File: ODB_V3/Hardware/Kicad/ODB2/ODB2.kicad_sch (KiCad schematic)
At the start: 95 parts, among them U1 STM32F412ZGTx, Y1 ABM8G-25.000MHZ-18-D2Y-T

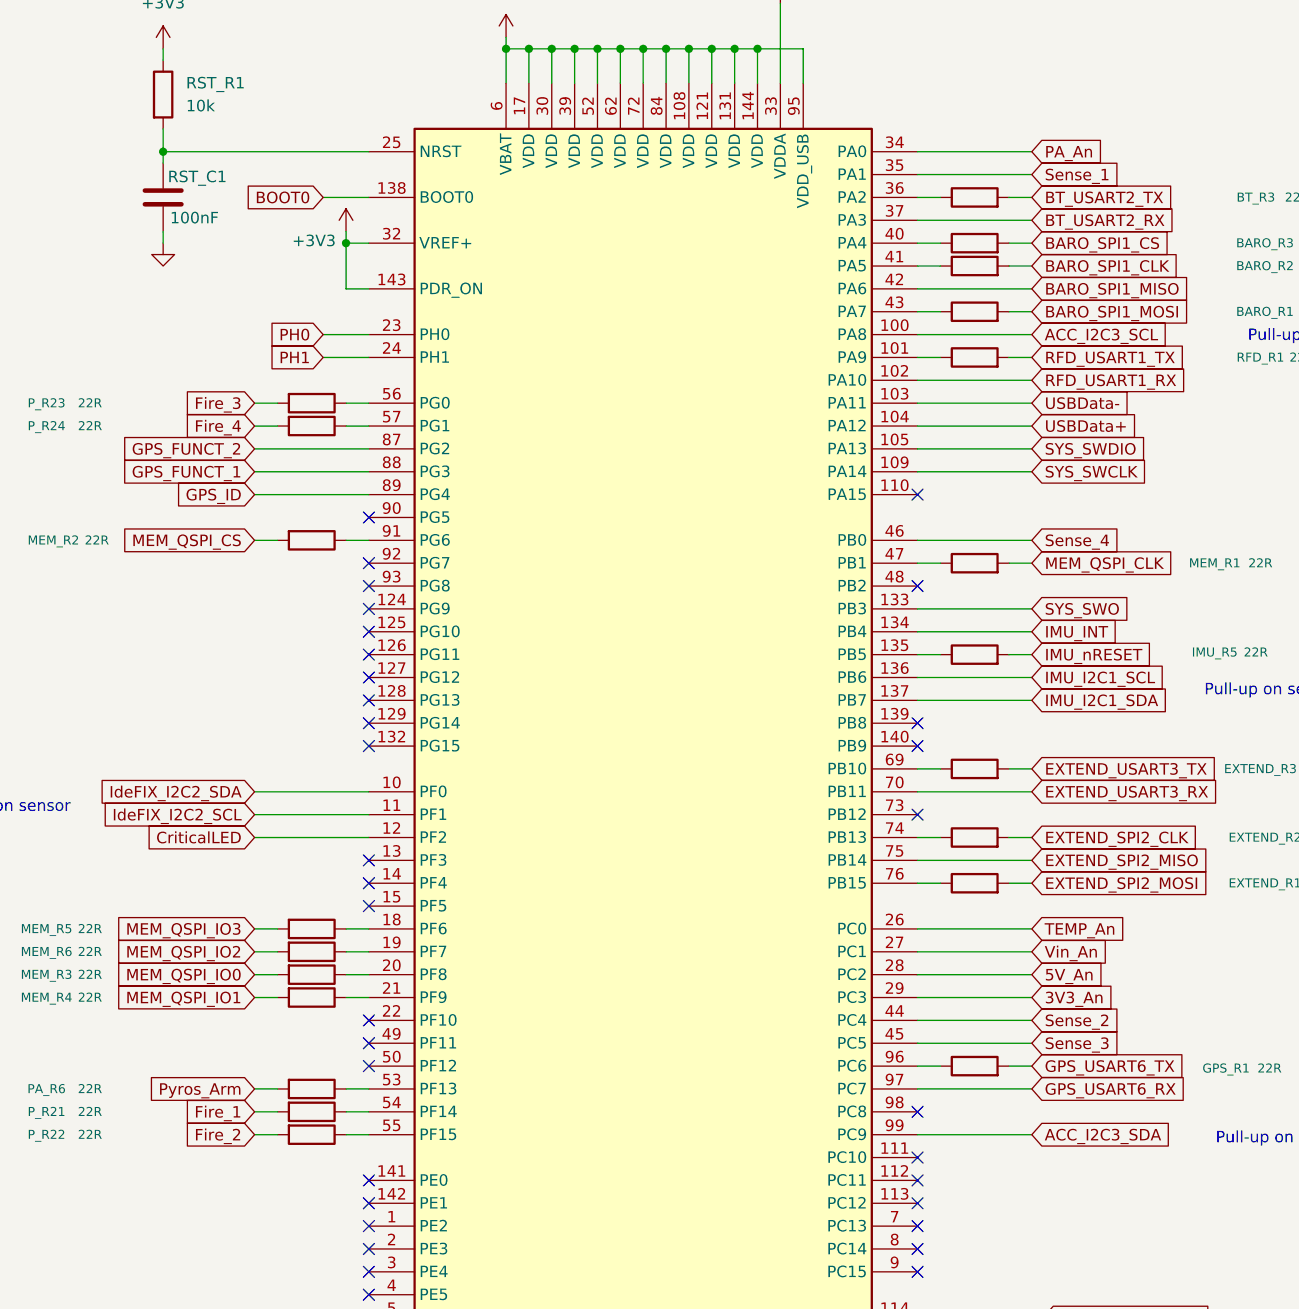
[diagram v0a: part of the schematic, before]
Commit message: WIP : routing pyros et interfaces communications
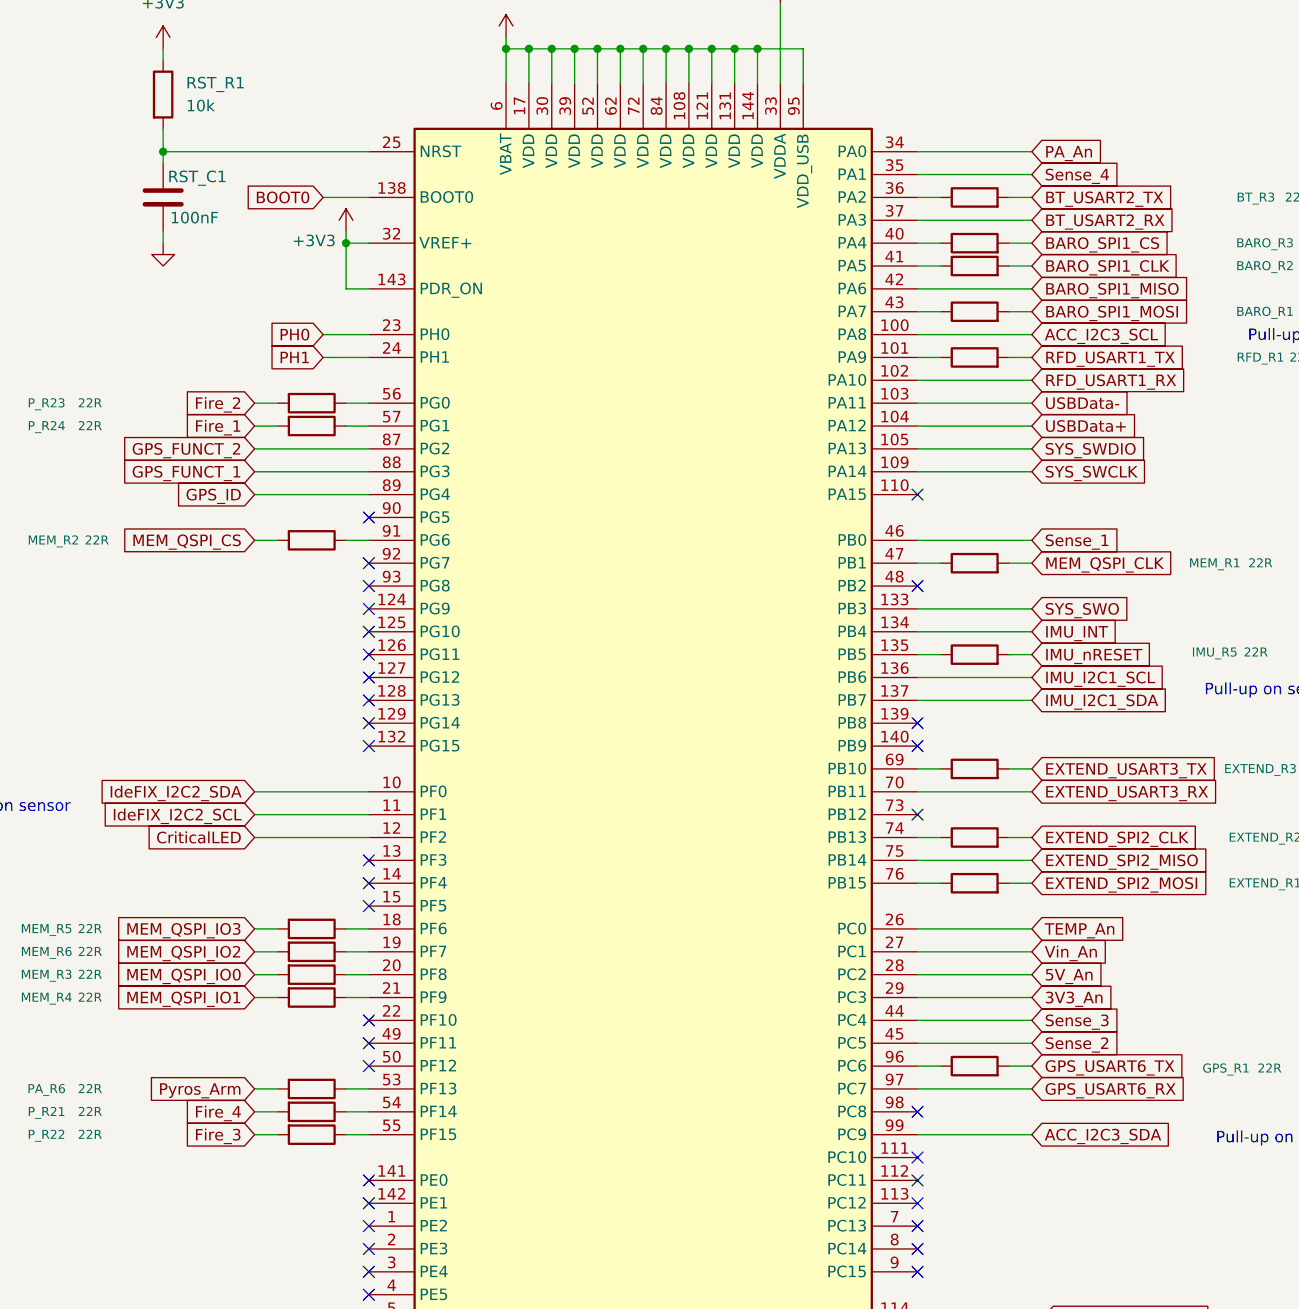
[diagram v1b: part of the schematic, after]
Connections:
- net Fire_1: now also P_R24.2; no longer P_R21.2
- net Fire_2: now also P_R23.2; no longer P_R22.2
- net Fire_3: now also P_R22.2; no longer P_R23.2
- net Fire_4: now also P_R21.2; no longer P_R24.2
- net Sense_1: now also U1.46 (PB0); no longer U1.35 (PA1)
- net Sense_2: now also U1.45 (PC5); no longer U1.44 (PC4)
- net Sense_3: now also U1.44 (PC4); no longer U1.45 (PC5)
- net Sense_4: now also U1.35 (PA1); no longer U1.46 (PB0)
